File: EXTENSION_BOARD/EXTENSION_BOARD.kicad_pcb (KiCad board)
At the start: 2 copper layers, 28 parts, among them IC1 Baro, IC2 ICM-20608-G, IC4 TeensyBuffer, J1 BATT, J3 PWM, J4 EXTOUT, U1 Teensy4.0, U2 COM-15809, U3 MOSBuzzer

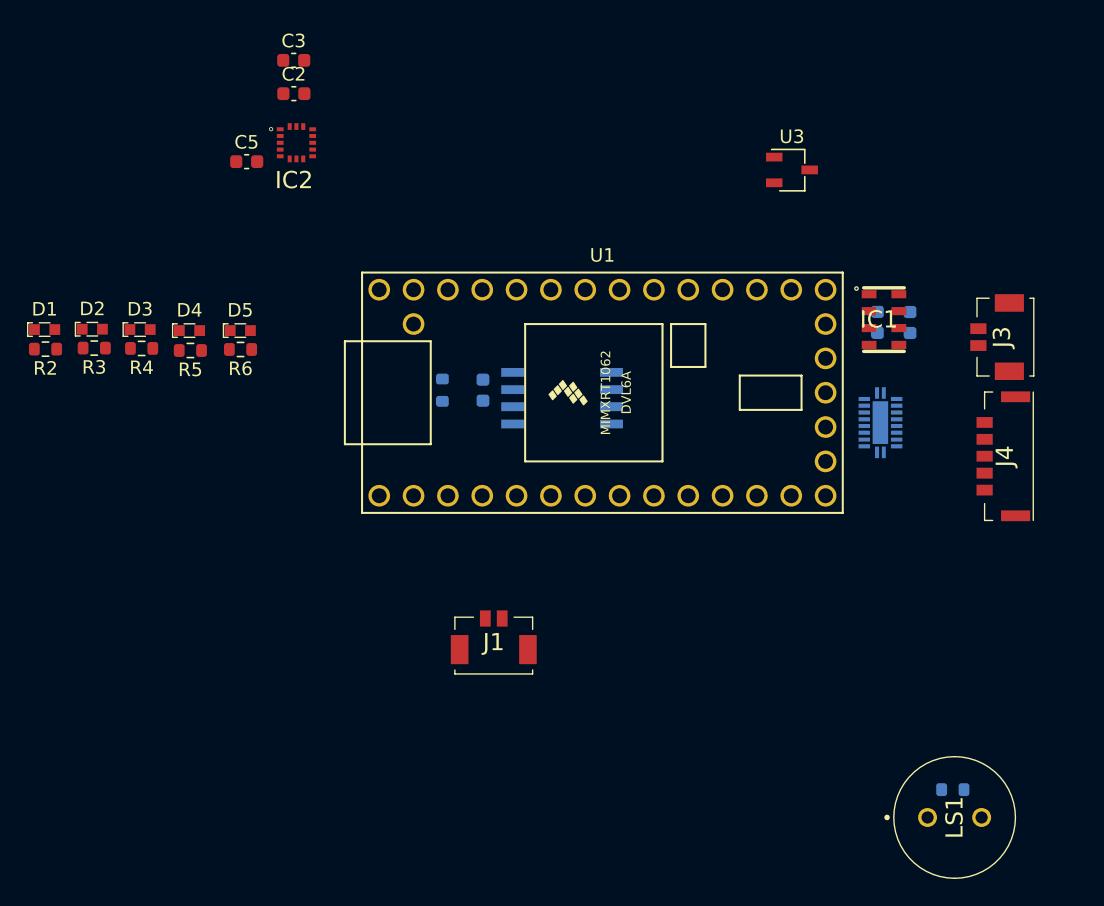
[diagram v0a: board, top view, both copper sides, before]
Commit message: Worked again
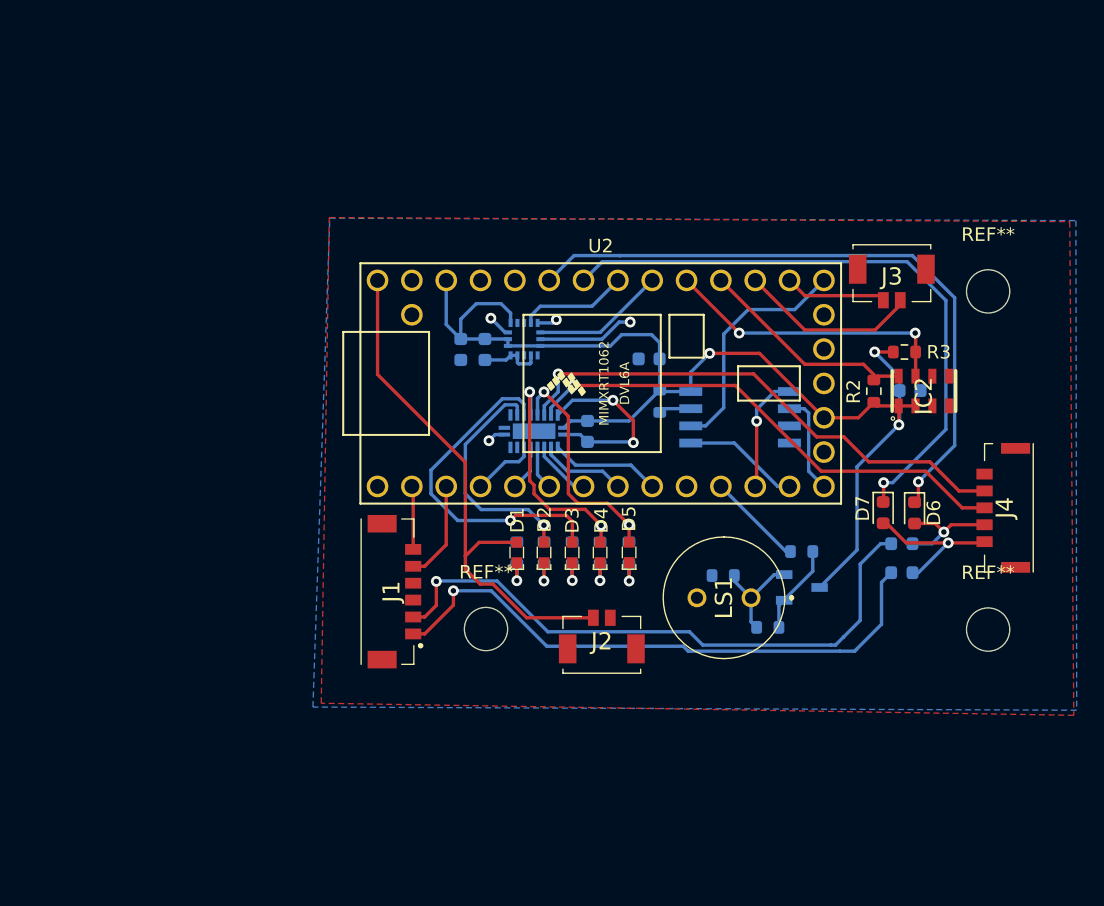
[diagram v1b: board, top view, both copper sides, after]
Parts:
- removed the C1 at (128.3, 83.9)
- removed the IC1 at (128.8, 83.7)
- removed the R1 at (133.9, 118.4)
- added AC1: Accel - H3LIS331DLTR, EXTENSION:LIS3DHTR, B.Cu at (102.2, 85.1)
- added D6: DIODE, Diode_SMD:D_0603_1608Metric, F.Cu at (131.1, 98.0)
- added D7: DIODE, Diode_SMD:D_0603_1608Metric, F.Cu at (128.7, 97.9)
- added D8: DIODE, Diode_SMD:D_0603_1608Metric, B.Cu at (130.1, 100.2)
- added D9: DIODE, Diode_SMD:D_0603_1608Metric, B.Cu at (130.1, 102.4)
- added J1: EXTIN, EXTENSION:5055670671, F.Cu at (92.4, 103.8)
- added R10: 330, Resistor_SMD:R_0603_1608Metric, B.Cu at (107.8, 100.9)
- added R11: 330, Resistor_SMD:R_0603_1608Metric, B.Cu at (109.9, 100.9)
- added R7: 500, Resistor_SMD:R_0603_1608Metric, B.Cu at (101.6, 100.9)
- added R8: 330, Resistor_SMD:R_0603_1608Metric, B.Cu at (103.7, 100.9)
- added R9: 330, Resistor_SMD:R_0603_1608Metric, B.Cu at (105.7, 100.9)
- added REF**: MountingHole_3.2mm_M3, MountingHole:MountingHole_3.2mm_M3, F.Cu at (99.4, 106.6)
- added REF**: MountingHole_3.2mm_M3, MountingHole:MountingHole_3.2mm_M3, F.Cu at (136.5, 106.6)
- added REF**: MountingHole_3.2mm_M3, MountingHole:MountingHole_3.2mm_M3, F.Cu at (136.5, 81.6)
- C2: moved to B.Cu
- C3: value 10nF -> 0.1uF; moved to B.Cu
- C4: value 2.2uF -> 10uF
- C5: value 0.47uF -> 0.1uF; moved to B.Cu
- IC1: renamed from IC4; value TeensyBuffer -> TeensyBuffer - 74AHCV541ABQX
- IC2: value ICM-20608-G -> Baro - MS561101BA03-50; footprint KRTEK_V2:PULL-BACK-QFN-16 -> KRTEK_V2:MS561101BA03-50
- LS1: value Buzzer -> Buzzer - CST-931AP
- R2: value 740 -> 10k
- R3: value 330 -> 10k
- R4: value 330 -> 1k; moved to B.Cu
- R5: value 330 -> 500; moved to B.Cu
- R6: value 330 -> 10k; moved to B.Cu
- U1: renamed from U2; value COM-15809 -> Flash - COM-15809
- U3: value MOSBuzzer -> MOSBuzzer - BSH105,235; moved to B.Cu
- moved R2 61.4 mm to (128.1, 89.0), turned to 270 degrees
- moved R3 59.9 mm to (130.3, 86.1)
- moved C2 50.6 mm to (130.7, 88.9), turned to 180 degrees
- moved IC2 49.9 mm to (131.8, 89.0), turned to 90 degrees
- moved R5 47.6 mm to (122.7, 100.8)
- moved R4 46.2 mm to (116.9, 102.6)
- moved R6 44.1 mm to (120.2, 106.4)
- moved D1 38.6 mm to (101.6, 100.9), turned to 90 degrees
- moved D2 37.3 mm to (103.7, 100.9), turned to 90 degrees
- moved D3 36.0 mm to (105.7, 100.9), turned to 90 degrees
- moved D4 34.5 mm to (107.8, 100.9), turned to 90 degrees
- moved D5 33.1 mm to (110.0, 100.9), turned to 90 degrees
- moved C5 32.2 mm to (106.9, 91.9), turned to 90 degrees
- moved C4 31.5 mm to (99.3, 85.9), turned to 270 degrees
- moved U3 30.9 mm to (122.7, 103.5)
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- renumbered C6 to C1, J1 to J2, R7 to R1, U1 to U2
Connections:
- net Net-(IC4-Pad11) renamed OUTFREE2
- net Net-(IC4-Pad12) renamed OUTFREE1
- net Net-(IC4-Pad8) renamed INFREE1
- net Net-(IC4-Pad9) renamed INFREE2
- C1 pad 1: 3V3 -> +3V3
- C2 pad 1: 3V3 -> GND
- C2 pad 2: GND -> +3V3
- C3 pad 1: 3V3 -> +3V3
- C4 pad 1: 3V3 -> +3V3
- C5 pad 2: Net-(C5-Pad2) -> +3V3
- D1 pad 2: VCC -> VIN
- IC1 pad 13: BUZZ2 -> YLED1
- IC1 pad 14: BUZZ1 -> YLED2
- IC1 pad 15: GLED2 -> GLED1
- IC1 pad 16: GLED1 -> GLED2
- IC1 pad 17: YLED2 -> BUZZ1
- IC1 pad 18: YLED1 -> BUZZ2
- IC1 pad 2: TYLED1 -> TBUZZ2
- IC1 pad 20: VIN -> +3V3
- IC1 pad 3: TYLED2 -> TBUZZ1
- IC1 pad 4: TGLED1 -> TGLED2
- IC1 pad 5: TGLED2 -> TGLED1
- IC1 pad 6: TBUZZ1 -> TYLED2
- IC1 pad 7: TBUZZ2 -> TYLED1
- IC2 pad 1: 3V3 -> +3V3
- IC2 pad 2: SCLK -> +3V3
- IC2 pad 3: SDI -> GND
- IC2 pad 4: SDO -> GND
- IC2 pad 5: CS_IMU -> GND
- IC2 pad 6: INT -> GND
- IC2 pad 7: RESV -> Baro_SDA
- IC2 pad 8: FSYNC -> Baro_SCLK
- J2 pad 1: GND -> VIN
- J2 pad 2: VIN -> GND
- J4 pad 1: PYRO1 -> GND
- J4 pad 2: PYRO2 -> BUZZ1
- J4 pad 3: BUZZ1 -> BUZZ2
- J4 pad 4: BUZZ2 -> OPYRO1
- J4 pad 5: GND -> OPYRO2
- R1 pad 1: 3V3 -> +3V3
- R2 pad 1: GND -> Baro_SCLK
- R2 pad 2: Net-(D1-Pad1) -> +3V3
- R3 pad 1: GND -> Baro_SDA
- R3 pad 2: Net-(D2-Pad1) -> +3V3
- R4 pad 1: GND -> Buzzer
- R4 pad 2: Net-(D3-Pad1) -> GND
- R5 pad 1: GND -> Net-(R5-Pad1)
- R5 pad 2: Net-(D4-Pad1) -> TBuzzer
- R6 pad 1: GND -> Net-(R5-Pad1)
- R6 pad 2: Net-(D5-Pad1) -> Buzzer
- U1 pad 8: 3V3 -> +3V3
- U2 pad 11: Net-(U1-Pad11) -> TBuzzer
- U2 pad 12: Net-(U1-Pad12) -> CS_FLASH
- U2 pad 13: Net-(U1-Pad13) -> MOSI
- U2 pad 14: Net-(U1-Pad14) -> MISO
- U2 pad 16: 3V3 -> +3V3
- U2 pad 2: Net-(U1-Pad2) -> HRX
- U2 pad 20: Net-(U1-Pad20) -> SCLK
- U2 pad 21: Net-(U1-Pad21) -> PWM1
- U2 pad 22: Net-(U1-Pad22) -> PWM2
- U2 pad 23: Net-(U1-Pad23) -> Baro_SCLK
- U2 pad 24: Net-(U1-Pad24) -> Baro_SDA
- U2 pad 25: Net-(U1-Pad25) -> Accel_SDA
- U2 pad 26: Net-(U1-Pad26) -> Accel_SCL
- U2 pad 27: Net-(U1-Pad27) -> TPyro2OUT
- U2 pad 28: Net-(U1-Pad28) -> TPyro1OUT
- U2 pad 3: Net-(U1-Pad3) (its old number) -> HTX
- U2 pad 31: 3V3 -> +3V3
- U2 pad 8: TBuzzer -> TBUZZ1
- U2 pad 9: Net-(U1-Pad9) -> TBUZZ2
- U3 pad 1: TBuzzer -> Net-(R5-Pad1)
- U3 pad 3: 3V3 -> +3V3
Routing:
- net +3V3: track 0.00 -> 85.9 mm, vias 0 -> 3
- net TPyro1OUT: track 0.00 -> 48.5 mm, vias 0 -> 1
- net TPyro2OUT: track 0.00 -> 45.8 mm, vias 0 -> 1
- net PYRO1: track 0.00 -> 45.0 mm, vias 0 -> 1
- net PYRO2: track 0.00 -> 43.5 mm, vias 0 -> 1
- net VIN: track 0.00 -> 39.2 mm
- net BUZZ1: track 0.00 -> 38.6 mm, vias 0 -> 1
- net BUZZ2: track 0.00 -> 37.0 mm, vias 0 -> 1
- net GND: track 0.00 -> 30.1 mm, vias 0 -> 6
- net YLED2: track 0.00 -> 24.9 mm, vias 0 -> 1
- net Baro_SDA: track 0.00 -> 21.7 mm, vias 0 -> 2
- net SCLK: track 0.00 -> 17.5 mm
- net YLED1: track 0.00 -> 17.4 mm, vias 0 -> 1
- net GLED2: track 0.00 -> 16.9 mm, vias 0 -> 2
- net GLED1: track 0.00 -> 16.6 mm, vias 0 -> 2
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- added copper zone on B.Cu, net GND
- added copper zone on F.Cu, net GND
